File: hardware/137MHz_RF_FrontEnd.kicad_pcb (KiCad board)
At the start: 2 copper layers, 75.8 x 40.1 mm, 39 parts, among them J1 Conn_Coaxial, J2 Conn_Coaxial, J3 Conn_01x02_Pin, Q1 AO3401A, U1 PGA-103, U2 TLV1117-50

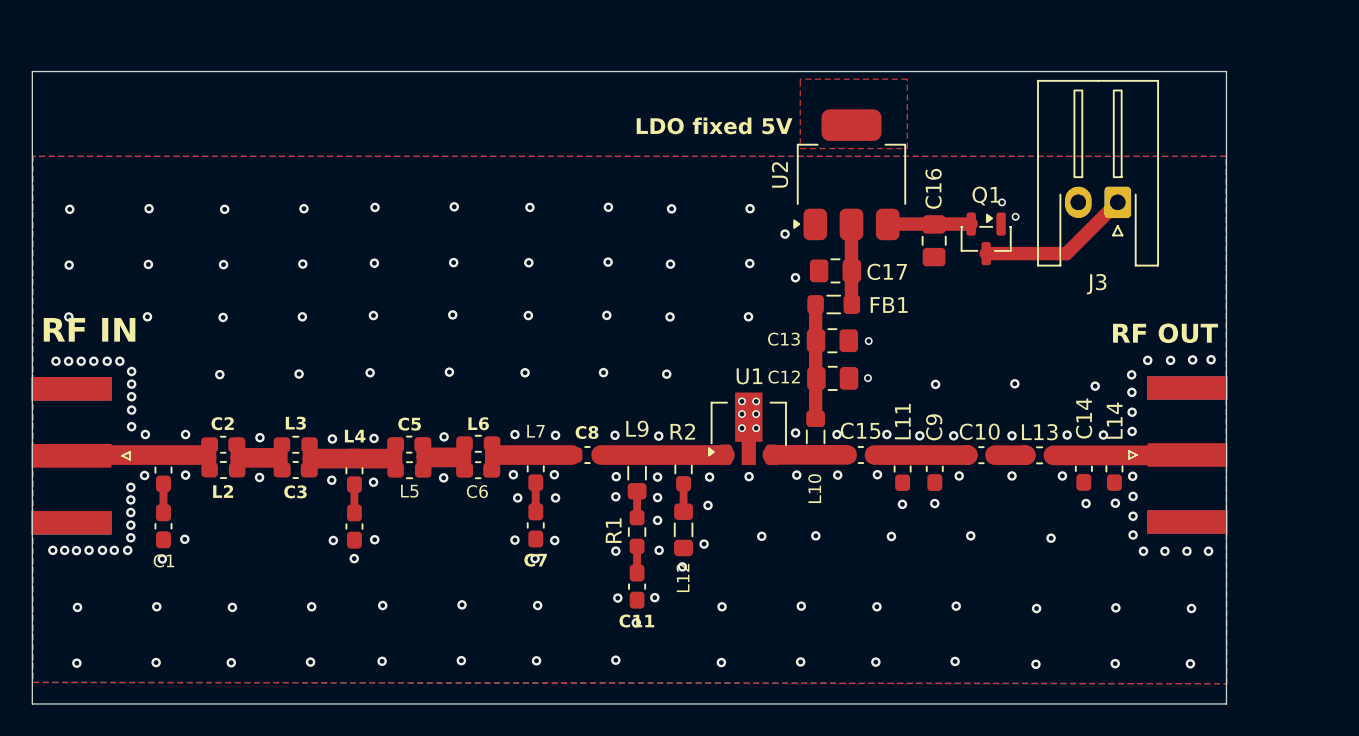
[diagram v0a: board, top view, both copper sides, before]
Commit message: update PCB
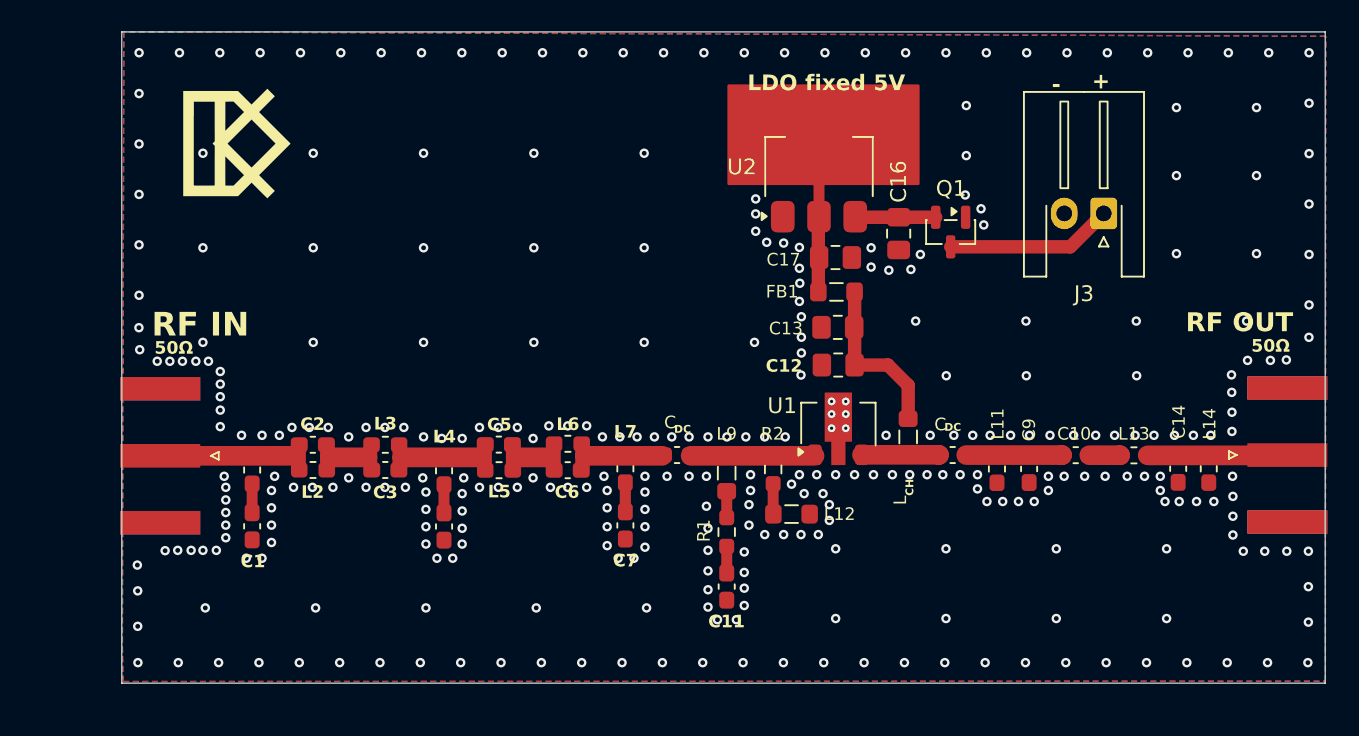
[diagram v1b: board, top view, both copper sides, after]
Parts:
- added -: -, LOGO, F.Cu at (127.6, 81.8)
- moved L12 6.92 mm to (162.9, 105.3), turned to 180 degrees
- moved J2 6.34 mm to (194.4, 101.5)
- moved C10 5.99 mm to (180.9, 101.6)
- moved C14 5.99 mm to (187.4, 102.4)
- moved L11 5.99 mm to (175.9, 102.4)
- moved L13 5.99 mm to (184.6, 101.6)
- moved L14 5.99 mm to (189.4, 102.4)
- moved C9 5.98 mm to (178.0, 102.4)
- moved L 5.87 mm to (170.3, 100.4)
- moved C 5.82 mm to (173.1, 101.5)
- moved C11 5.69 mm to (158.8, 109.9)
- moved C2 5.69 mm to (132.5, 100.9)
- moved C3 5.69 mm to (137.1, 102.5)
- moved C4 5.69 mm to (140.8, 106.1)
- moved C5 5.69 mm to (144.3, 100.9)
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- renumbered C15 to C, L10 to L
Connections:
- U2 pad 4: (no net) -> Net-(U2-VO)
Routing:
- net Net-(U2-VO): track 5.09 -> 11.0 mm
- net Net-(C12-Pad1): track 7.25 -> 10.7 mm
- net Net-(J3-Pin_1): track 9.70 -> 10.6 mm
- net GND: vias 186 -> 334
- removed copper zone on F.Cu, net Net-(U2-VO)
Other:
- board size 75.8 x 40.1 mm -> 76.4 x 41.3 mm
- board text added: "+"
- board text added: "-"
- board text added: "50Ω"
- board text added: "C"
- board text added: "CH"
- board text added: "DC"
